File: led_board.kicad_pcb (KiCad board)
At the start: 2 copper layers, 185 x 120 mm, 24 parts, among them J1 Conn_Coaxial, J2 Conn_Coaxial, J3 Conn_Coaxial, J4 Conn_Coaxial

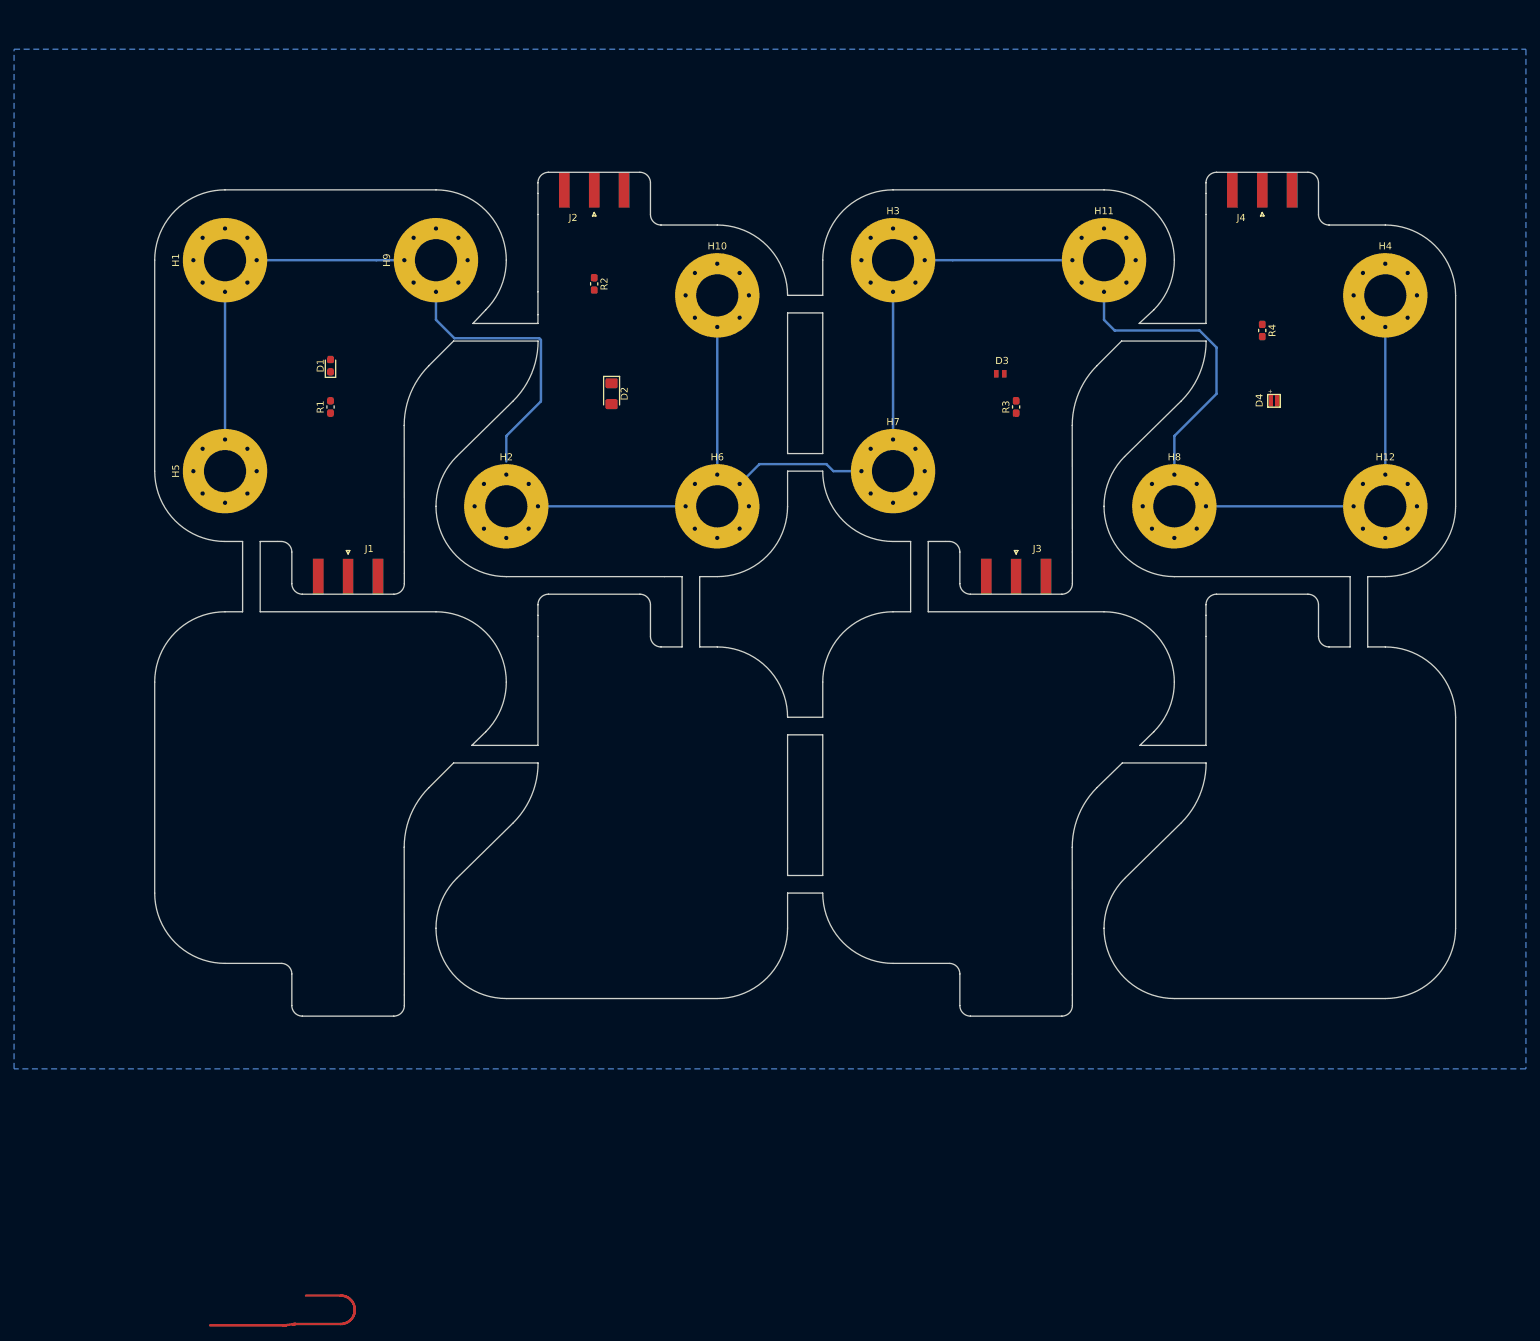
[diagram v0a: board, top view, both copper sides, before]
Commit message: fcu pour
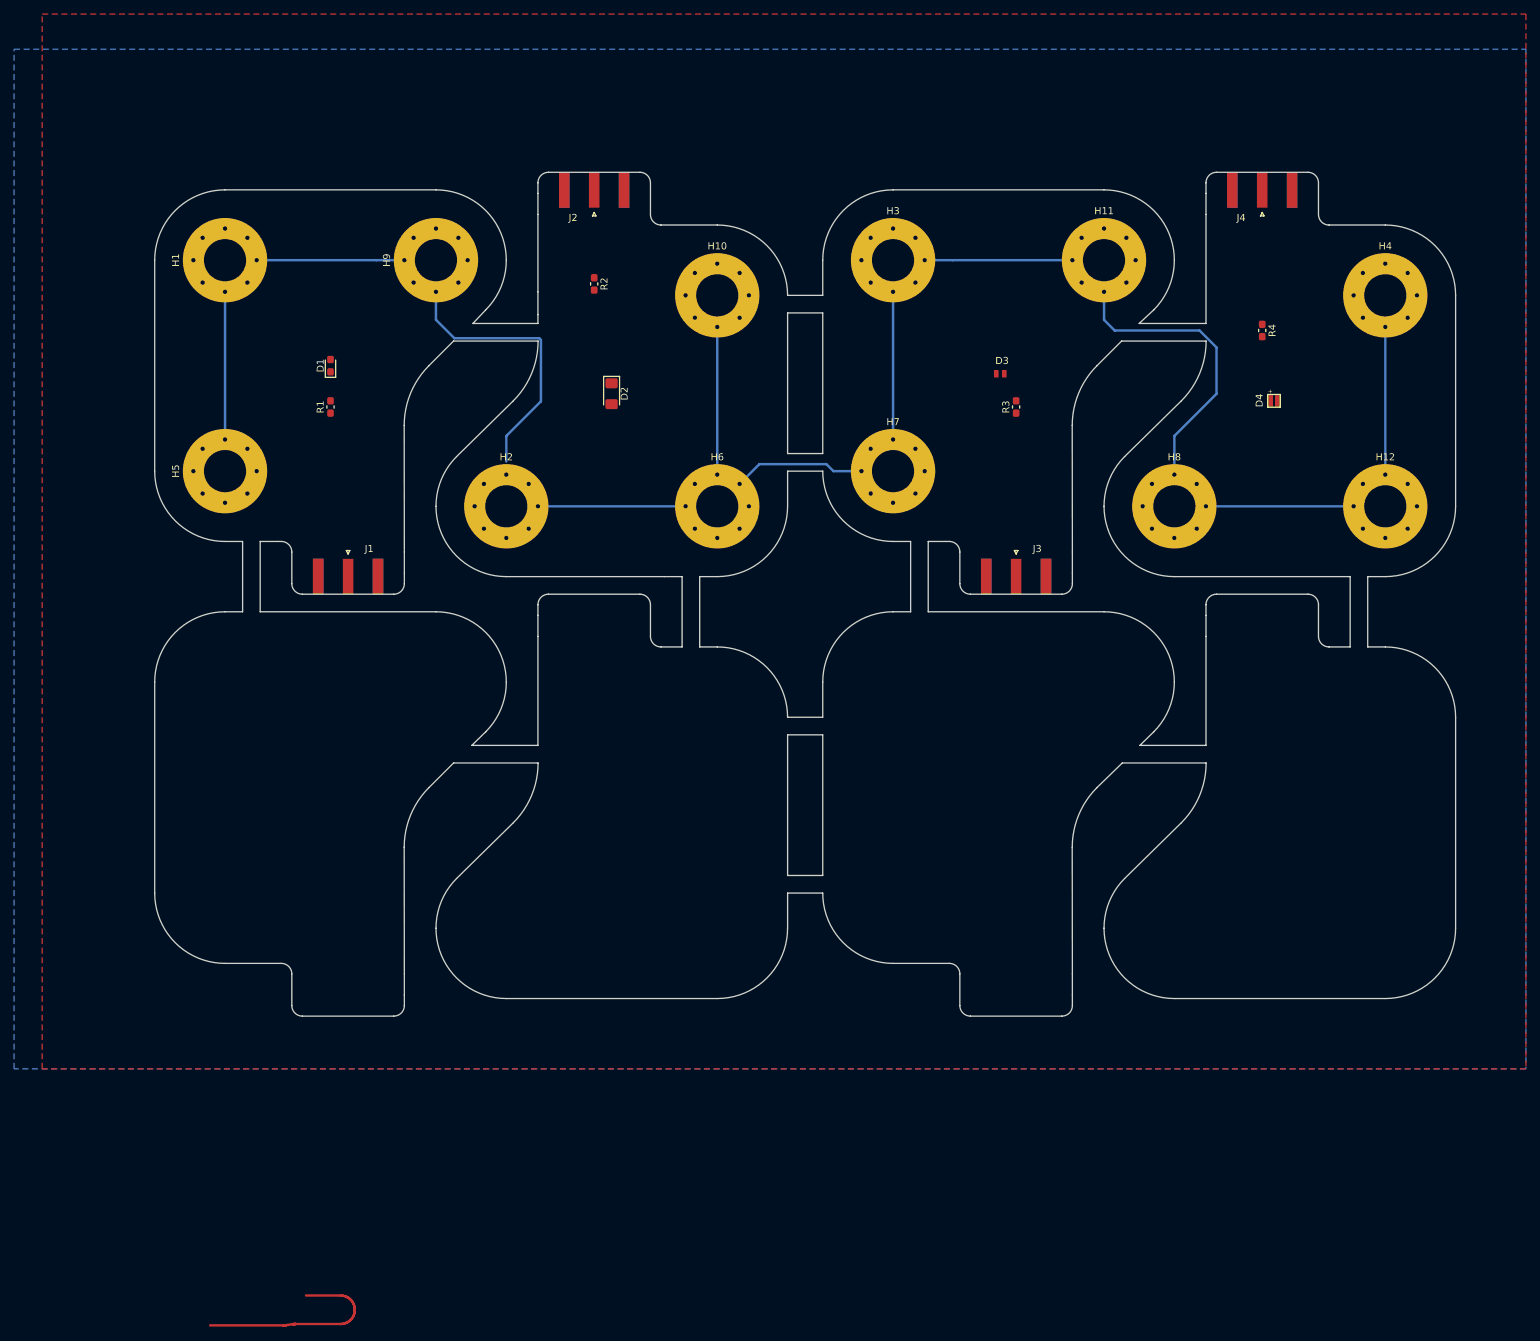
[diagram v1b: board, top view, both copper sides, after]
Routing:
- added copper zone on F.Cu, net GND
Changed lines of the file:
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@@
   )
   (setup
-    (last_trace_width 0.349)
+    (last_trace_width 0.25)
     (user_trace_width 0.349)
     (trace_clearance 0.2)
@@
   (gr_line (start 65.479186 63.5) (end 65.5 81.5) (layer Edge.Cuts) (width 0.05))
   (gr_arc (start 48 81.5) (end 49.5 81.5) (angle -90) (layer Edge.Cuts) (width 0.05))
-  (segment (start 61.514719 40) (end 40 40) (width 0.349) (layer B.Cu) (net 10))
-  (segment (start 70 40) (end 61.514719 40) (width 0.349) (layer B.Cu) (net 10))
-  (segment (start 40 40) (end 40 70) (width 0.349) (layer B.Cu) (net 10))
-  (segment (start 84.921817 51.333897) (end 84.921817 60.078183) (width 0.349) (layer B.Cu) (net 10))
-  (segment (start 84.68841 51.10049) (end 84.921817 51.333897) (width 0.349) (layer B.Cu) (net 10))
-  (segment (start 72.615209 51.10049) (end 84.68841 51.10049) (width 0.349) (layer B.Cu) (net 10))
-  (segment (start 70 40) (end 70 48.485281) (width 0.349) (layer B.Cu) (net 10))
-  (segment (start 70 48.485281) (end 72.615209 51.10049) (width 0.349) (layer B.Cu) (net 10))
-  (segment (start 84.921817 60.078183) (end 80 65) (width 0.349) (layer B.Cu) (net 10))
-  (segment (start 80 65) (end 80 68.625499) (width 0.349) (layer B.Cu) (net 10))
   (segment (start 48.584912 191.461938) (end 48.609713 191.459153) (width 0.349) (layer F.Cu) (net 5))
   (segment (start 48.609713 191.459153) (end 48.634488 191.456146) (width 0.349) (layer F.Cu) (net 5))
@@
   (segment (start 57.217366 191.131759) (end 57.394793 191.047842) (width 0.349) (layer F.Cu) (net 5))
   (segment (start 58.41357 189.67418) (end 58.442369 189.480034) (width 0.349) (layer F.Cu) (net 5))
+  (segment (start 61.514719 40) (end 40 40) (width 0.349) (layer B.Cu) (net 10))
+  (segment (start 70 40) (end 61.514719 40) (width 0.349) (layer B.Cu) (net 10))
+  (segment (start 40 40) (end 40 70) (width 0.349) (layer B.Cu) (net 10))
+  (segment (start 84.921817 51.333897) (end 84.921817 60.078183) (width 0.349) (layer B.Cu) (net 10))
+  (segment (start 84.68841 51.10049) (end 84.921817 51.333897) (width 0.349) (layer B.Cu) (net 10))
+  (segment (start 72.615209 51.10049) (end 84.68841 51.10049) (width 0.349) (layer B.Cu) (net 10))
+  (segment (start 70 40) (end 70 48.485281) (width 0.349) (layer B.Cu) (net 10))
+  (segment (start 70 48.485281) (end 72.615209 51.10049) (width 0.349) (layer B.Cu) (net 10))
+  (segment (start 84.921817 60.078183) (end 80 65) (width 0.349) (layer B.Cu) (net 10))
+  (segment (start 80 65) (end 80 68.625499) (width 0.349) (layer B.Cu) (net 10))
   (segment (start 80 75) (end 110 75) (width 0.349) (layer B.Cu) (net 10))
   (segment (start 110 75) (end 110 45) (width 0.349) (layer B.Cu) (net 10))
@@
       )
     )
+  )
+  (zone (net 10) (net_name GND) (layer F.Cu) (hatch edge 0.508)
+    (connect_pads (clearance 0.508))
+    (min_thickness 0.254)
+    (fill yes (arc_segments 32) (thermal_gap 0.508) (thermal_bridge_width 0.508))
+    (polygon
+      (pts
+        (xy 225 155) (xy 14 155) (xy 14 5) (xy 225 5)
+      )
+    )
